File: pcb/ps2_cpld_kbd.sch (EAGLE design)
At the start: 35 parts, among them J1 AVR ISP, J2 JTAG, J3 Emulated Mechanical Keyboard, J4 VCC GND, J5 PS/2, U1 ATMEGA328, U2 EPM7128, Y1 16MHz

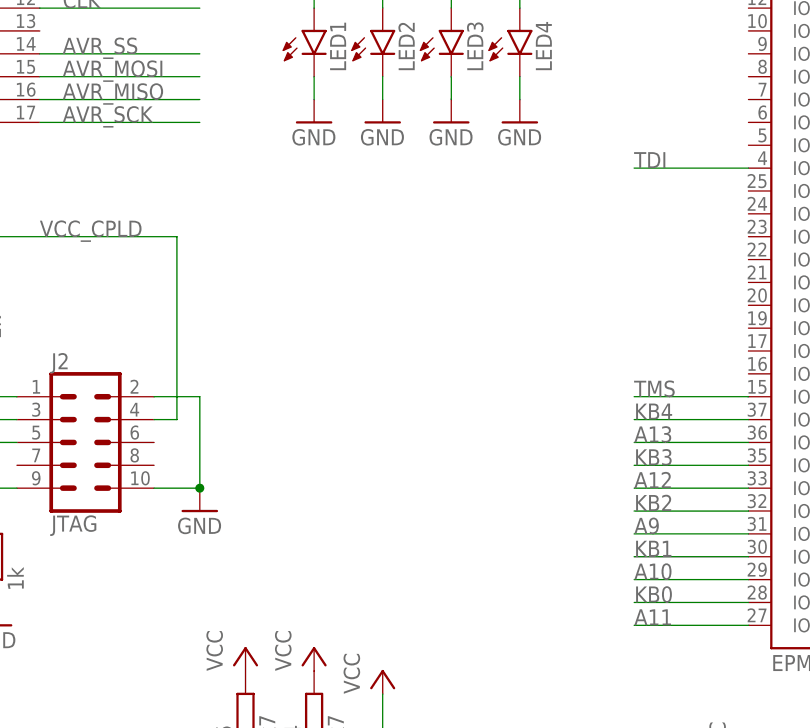
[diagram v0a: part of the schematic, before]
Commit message: new board v1.2 with fixes
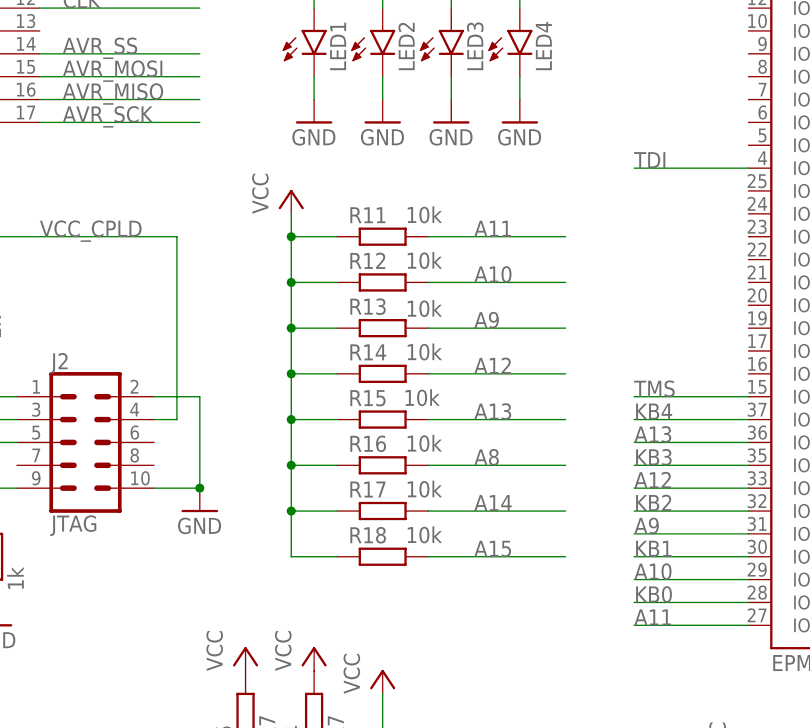
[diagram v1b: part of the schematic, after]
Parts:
- added R11, R12, R13, R14, R15, R16, R17, R18: 10k, rcl:R-EU_R0805
- J4: device pinhead:PINHD-1X2 -> pinhead-mod:PINHD-1X2
- JP1: device jumper:JP1Q -> jumper-mod:JP1Q
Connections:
- net A10: now also R12.2
- net A11: now also R11.2
- net A12: now also R14.2
- net A13: now also R15.2
- net A14: now also R17.2
- net A15: now also R18.2
- net A8: now also R16.2
- net A9: now also R13.2
- net VCC: now also R11.1, R12.1, R13.1, R14.1, R15.1, R16.1, R17.1, R18.1
